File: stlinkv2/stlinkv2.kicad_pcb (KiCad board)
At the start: 2 copper layers, 80 x 45.7 mm, 86 parts, among them J1 STLSWD, J2 JTAG, J3 SWD, J4 CLONE, J5 DBG_UART, J6 STM8, J7 POWER, J8 POWER, J9 USB_B_Mini, SW1 EXRERNAL POWER, U1 STM32F103CBTx, U2 74LVCC3245, U3 LD3985M33R_SOT23, U4 USBLC6-2, U5 ADUM3160, Y1 8MHz

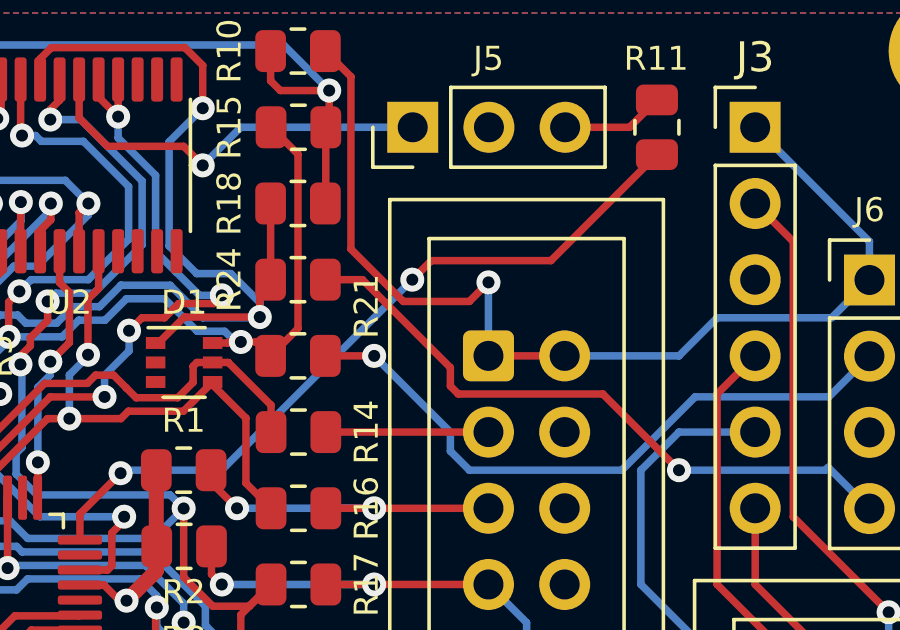
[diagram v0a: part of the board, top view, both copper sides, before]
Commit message: some update
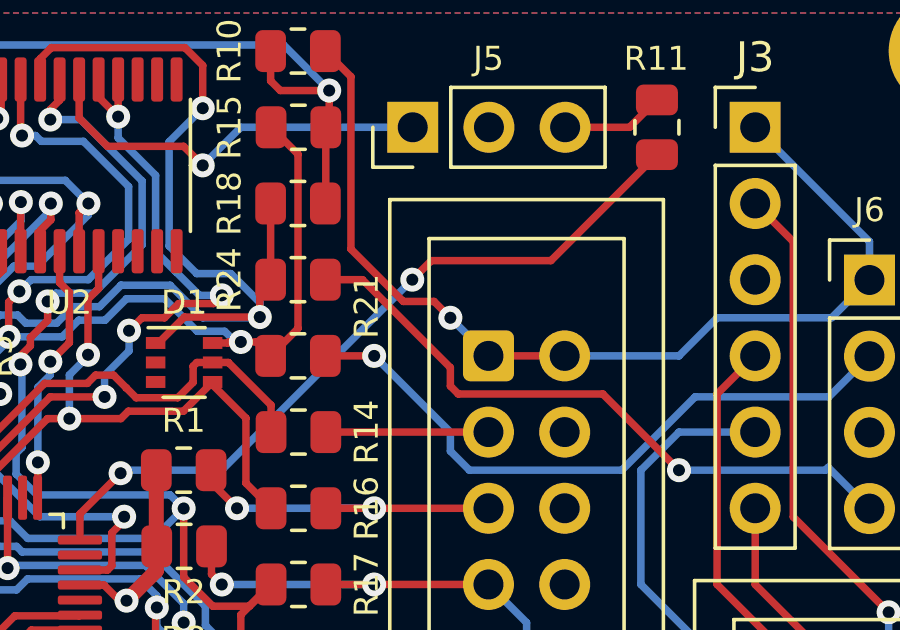
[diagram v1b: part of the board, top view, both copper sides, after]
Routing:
- net V_TGT: track 35.4 -> 33.4 mm
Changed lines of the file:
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@@
   (segment (start 62.68 47.819293) (end 62.68 35.13) (width 0.25) (layer "B.Cu") (net 34))
   (segment (start 84.789695 36.285) (end 83.045 34.540305) (width 0.25) (layer "F.Cu") (net 35))
-  (segment (start 86.9945 36.285) (end 84.789695 36.285) (width 0.25) (layer "F.Cu") (net 35))
-  (segment (start 87.63 35.6495) (end 86.9945 36.285) (width 0.25) (layer "F.Cu") (net 35))
-  (segment (start 87.63 38.1) (end 90.17 38.1) (width 0.25) (layer "F.Cu") (net 35))
   (segment (start 83.045 28.7925) (end 82.1925 27.94) (width 0.25) (layer "F.Cu") (net 35))
   (segment (start 83.045 34.540305) (end 83.045 28.7925) (width 0.25) (layer "F.Cu") (net 35))
-  (via (at 87.63 35.6495) (size 0.8) (drill 0.4) (layers "F.Cu" "B.Cu") (net 35))
+  (segment (start 87.63 38.1) (end 90.17 38.1) (width 0.25) (layer "F.Cu") (net 35))
+  (segment (start 86.36 36.83) (end 85.815 36.285) (width 0.25) (layer "F.Cu") (net 35))
+  (segment (start 85.815 36.285) (end 84.789695 36.285) (width 0.25) (layer "F.Cu") (net 35))
+  (via (at 86.36 36.83) (size 0.8) (drill 0.4) (layers "F.Cu" "B.Cu") (net 35))
   (segment (start 96.52 30.48) (end 100.33 34.29) (width 0.25) (layer "B.Cu") (net 35))
   (segment (start 93.98 38.1) (end 95.25 36.83) (width 0.25) (layer "B.Cu") (net 35))
@@
   (segment (start 90.17 38.1) (end 93.98 38.1) (width 0.25) (layer "B.Cu") (net 35))
   (segment (start 100.33 34.29) (end 100.33 35.57) (width 0.25) (layer "B.Cu") (net 35))
-  (segment (start 87.63 35.6495) (end 87.63 38.1) (width 0.25) (layer "B.Cu") (net 35))
+  (segment (start 86.36 36.83) (end 87.63 38.1) (width 0.25) (layer "B.Cu") (net 35))
   (segment (start 83.82 38.1) (end 82.1925 38.1) (width 0.25) (layer "F.Cu") (net 36))
   (via (at 83.82 38.1) (size 0.8) (drill 0.4) (layers "F.Cu" "B.Cu") (net 36))
